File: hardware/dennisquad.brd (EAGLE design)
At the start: 25 x 25 mm, 47 parts, among them U1 MPU-9250, U10 DRV8839, U2 NRF52832_QFN48, U3 DRV8839, U4 LPS25HB, U5 MCP1700T-3302E/MAY, X1 8Y-32.000MAAV-T, X2 CRYSTAL.ABS07

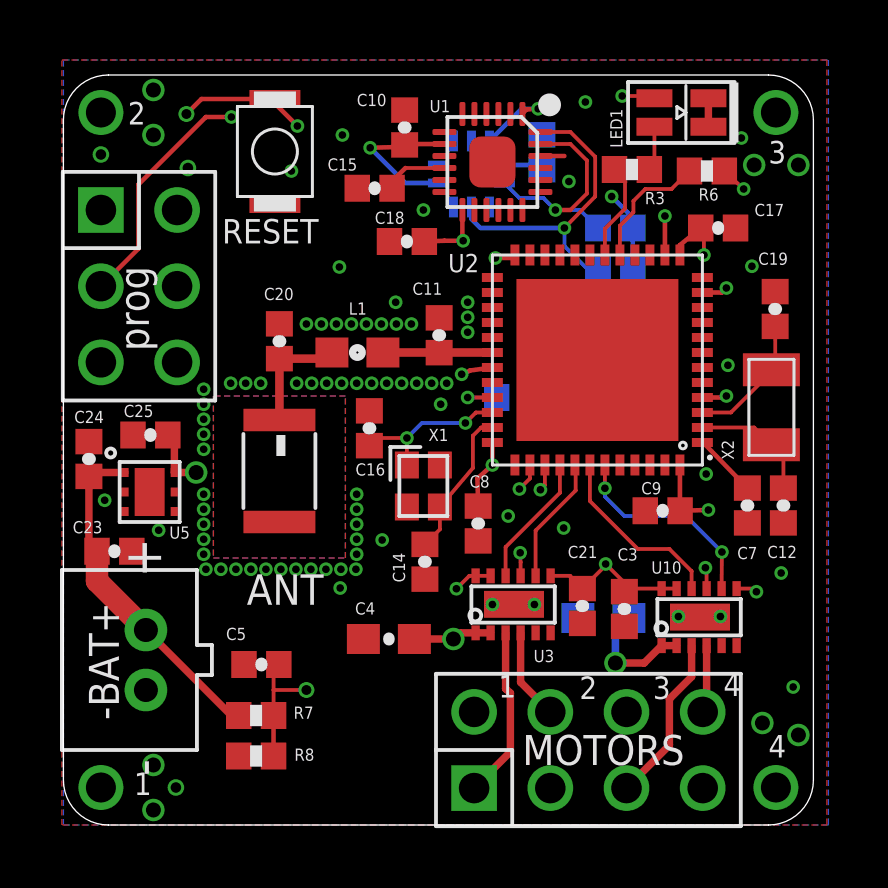
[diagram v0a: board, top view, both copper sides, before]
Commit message: Version 0.9
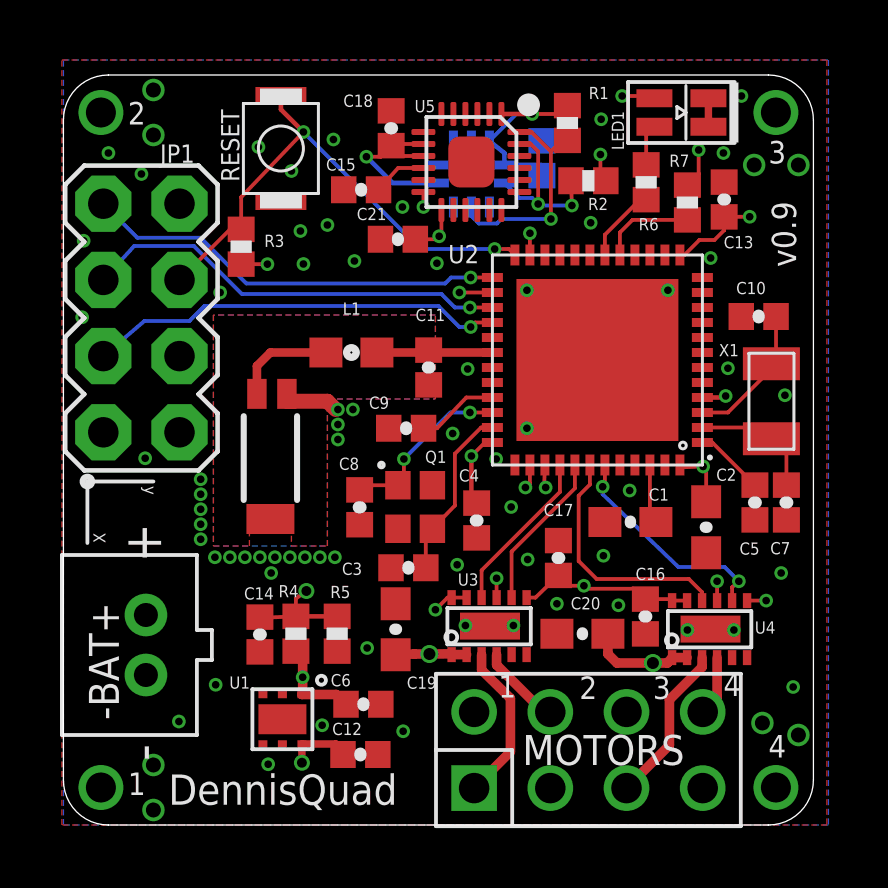
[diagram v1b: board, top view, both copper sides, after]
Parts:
- removed ANT: ANTENNA-BLE, NordicSemi:BTE
- removed C23, C25: 2.2uF, SparkFun-Capacitors:0402-CAP
- removed C24: 0.47uF, SparkFun-Capacitors:0402-CAP
- removed CN3: (no value), adafruit:JST-PH-2-THM
- removed R8: 4k7, SparkFun-Resistors:0402-RES
- removed U$2: FIDUCIAL, jaw:FIDUCIAL
- removed U10: DRV8839, jseng:PWSON-N12
- removed X2: CRYSTAL.ABS07, abracon:ABS07
- added C1: 1.0uF, SparkFun-Capacitors:0603-CAP
- added C2: 4.7pF, SparkFun-Capacitors:0603-CAP
- added JP1: (no value), SparkFun-Connectors:2X4
- added Q1: FA-128, crystal:FA-128
- added R4, R5: 4k7, SparkFun-Resistors:0402-RES
- added U6: LPS25HB, jaw:HLGA10L
- C10: value 10nF -> 8pF
- C11: value 0.8pf -> 0.8pF
- C12: value 8pF -> 2.2uF
- C13: value 100pf -> 0.1uF
- C14, C16: value 12pf -> 0.1uF
- C17: value 100nf -> 0.1uF
- C18: value 0.1uF -> 10000pF
- C19: value 8pF -> 10uF; device SparkFun-Capacitors:0402-CAP -> SparkFun-Capacitors:0603-CAP
- C20: value 1.2pf -> 10uF; device SparkFun-Capacitors:0402-CAP -> SparkFun-Capacitors:0603-CAP
- C21, C5: value .1u -> 0.1uF
- C22, C4: value 10uF -> 0.1uF; device SparkFun-Capacitors:0603-CAP -> SparkFun-Capacitors:0402-CAP
- C3: value .1u -> 16pF
- C6: value .1u -> 2.2uF
- C7: value 100nf -> 8pF
- C8: value 100nf -> 16pF
- C9: value 4.7pf -> 100pF
- CN1: device jaw:HEADER-2X04-THM -> adafruit:JST-PH-2-THM
- CN2: device jaw:HEADER-3X2-PTH -> jaw:HEADER-2X04-THM
- R7: value 4k7 -> 1k
- U$1: value ROBOTMAN-LOGO -> ANTENNA-W3008C; device jaw:ROBOTMAN-LOGO -> SparkFun-RF:ANTENNA-W3008C
- U1: value MPU-9250 -> MCP1700T-3302E/MAY; device template:LEAD-QFN24 -> wrea:6-VDFN
- U4: value LPS25HB -> DRV8839; device jaw:HLGA10L -> jseng:PWSON-N12
- U5: value MCP1700T-3302E/MAY -> MPU-9250; device wrea:6-VDFN -> template:LEAD-QFN24
- X1: value 8Y-32.000MAAV-T -> CRYSTAL.ABS07; device crystals:TXC-8Y -> abracon:ABS07
- moved CN2 24.2 mm to (17.5, 2.50), turned to 0 degrees
- moved R7 22.3 mm to (20.8, 20.8), turned to 270 degrees
- moved U1 19.9 mm to (7.30, 3.52), turned to 180 degrees
- moved C6 19.3 mm to (10.0, 4.03), flipped to the top, turned to 0 degrees
- moved U4 17.3 mm to (20.8, 5.90), flipped to the top
- moved C5 17.3 mm to (23.1, 10.8), turned to 270 degrees
- moved C19 16.6 mm to (11.1, 6.53)
- moved C12 16.4 mm to (9.90, 2.35), turned to 180 degrees
- moved C22 15.5 mm to (15.9, 22.2), turned to 90 degrees
- moved U5 15.4 mm to (13.6, 22.1)
- moved CN1 15.2 mm to (2.75, 6.00), turned to 90 degrees
- moved C20 14.0 mm to (17.3, 6.38), turned to 180 degrees
- moved C21 13.7 mm to (11.2, 19.5), turned to 0 degrees
- moved C10 13.4 mm to (23.2, 16.9), turned to 180 degrees
- moved R3 13.3 mm to (5.92, 19.3), turned to 270 degrees
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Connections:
- removed net AD0/SDO: U1.9
- removed net BOOT0: CN2.5
- removed net INT: U1.12
- new net IMU_INT: U2.23, U5.12
- new net N$22: C1.1, U2.46
- new net SWDCK: JP1.8, U2.25
- new net SWDIO: JP1.7, U2.26
- net AIN0: now also C14.1, R4.1, R5.2; no longer C5.1, R7.1, R8.2
- net GND: now also C1.2, C12.1, C16.2, C17.1, C18.2, C2.1, C20.2, C4.1, C9.2, CN2.3, CN2.6, CN2.7, JP1.2, Q1.2, Q1.4, R5.1, U$1.GND, U$1.GROUND, U1.3, U1.P$1, U4.GND, U4.P$5, U4.P$6, U5.11, U5.18, U5.19, U5.20, U5.21, U5.22, U5.7, U6.5, U6.8, U6.9; no longer C12.2, C16.1, C17.2, C18.1, C20.1, C23.2, C24.1, C25.1, C4.2, C9.1, CN1.3, CN1.6, CN1.7, CN3.2, R8.1, U1.11, U1.18, U1.20, U1.21, U1.22, U1.7, U10.GND, U10.P$5, U10.P$6, U4.5, U4.8, U4.9, U5.3, U5.P$1, X1.2, X1.4
- net IOA2: now also U4.P$9; no longer U10.P$9
- net IOA3: now also U4.P$11; no longer U10.P$11
- net LED1: now also R6.2; no longer R3.2
- net LED2: now also R7.2; no longer R6.2
- net N$12: now also U5.10; no longer U1.10
- net N$13: now also C7.1, X1.1; no longer C12.1, X2.1
- net N$14: now also R6.1; no longer R3.1
- net N$15: now also R7.1; no longer R6.1
- net N$16: now also CN2.1; no longer CN1.1
- net N$17: now also CN2.4; no longer CN1.4
- net N$18: now also U$1.FEED; no longer ANT.FP, C20.2
- net N$19: now also CN2.5, U4.P$3; no longer CN1.5, U10.P$3
- net N$20: now also CN2.8, U4.P$4; no longer CN1.8, U10.P$4
- net N$21: now also C10.1, X1.2; no longer C19.1, X2.2
- net N$26: now also C5.1; no longer C7.1
- net N$28: now also C9.1; no longer C13.1
- net N$30: now also C8.2, Q1.1; no longer C16.2, X1.1
- net N$31: now also C3.1, Q1.3; no longer C14.1, X1.3
- net RESET: now also JP1.5, R3.1; no longer CN2.6
- net RX: now also JP1.6, U2.27; no longer CN2.3, U2.14
- net SCL: now also U5.23, U6.2; no longer U1.23, U4.2
- net SDA: now also U5.24, U6.4; no longer U1.24, U4.4
- net TX: now also JP1.4, U2.28; no longer CN2.4, U2.11
- net VCC: now also C12.2, C13.1, C16.1, C17.2, C18.1, C2.2, C22.1, C4.2, JP1.1, R3.2, U1.6, U4.P$10, U4.P$12, U4.P$7, U4.P$8, U5.1, U5.13, U5.8, U5.9, U6.1, U6.10, U6.6; no longer C10.1, C17.1, C18.2, C25.2, C3.1, C6.1, C8.2, C9.2, U1.1, U1.13, U1.8, U10.P$10, U10.P$12, U10.P$7, U10.P$8, U4.1, U4.10, U4.6, U5.6
- net VCCM: now also C19.1, C20.1, C6.1, CN1.1, R4.2, U1.1, U4.P$1, U4.P$2; no longer C22.1, C23.1, C24.2, C4.1, CN2.1, CN3.1, R7.2, U10.P$1, U10.P$2, U5.1
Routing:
- net VCCM: track 48.7 -> 28.6 mm, vias 2 -> 3
- net TX: track 28.3 -> 14.0 mm
- net SWDCK: track 0.00 -> 14.2 mm, vias 0 -> 1
- net SWDIO: track 0.00 -> 11.7 mm, vias 0 -> 1
- net RX: track 25.7 -> 14.3 mm, vias 2 -> 1
- net RESET: track 23.0 -> 17.1 mm, vias 3 -> 2
- net IMU_INT: track 0.00 -> 5.14 mm, vias 0 -> 2
- net SDA: track 21.3 -> 18.4 mm
- net SCL: track 19.6 -> 16.9 mm, vias 2 -> 3
- net IOA2: track 6.14 -> 8.18 mm
- net N$22: track 0.00 -> 1.98 mm
- net VCC: track 33.5 -> 35.4 mm, vias 13 -> 14
- net N$15: track 7.32 -> 5.90 mm
- net AIN0: track 23.2 -> 21.8 mm
- net LED2: track 4.27 -> 3.17 mm
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- added copper zone on layer 2, net GND
- added copper zone on layer 15, net VCC
- removed copper zone on layer 15, net GND
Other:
- board text added: "3.3v"
- board text added: "DennisQuad"
- board text added: "GND"
- board text added: "RESET"
- board text added: "RX"
- board text added: "SWDCK"
- board text added: "SWDIO"
- board text added: "TX"
- board text added: "v0.9"
- board text added: "y"
- board text removed: "JAW 2015-10"
- board text removed: "minicopter Rev. 1"
- board text removed: "prog"
- board text removed: "www.tcp4me.com"
